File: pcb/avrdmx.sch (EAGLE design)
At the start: 15 parts, among them U1 ARDUINO_SHIELDLABEL

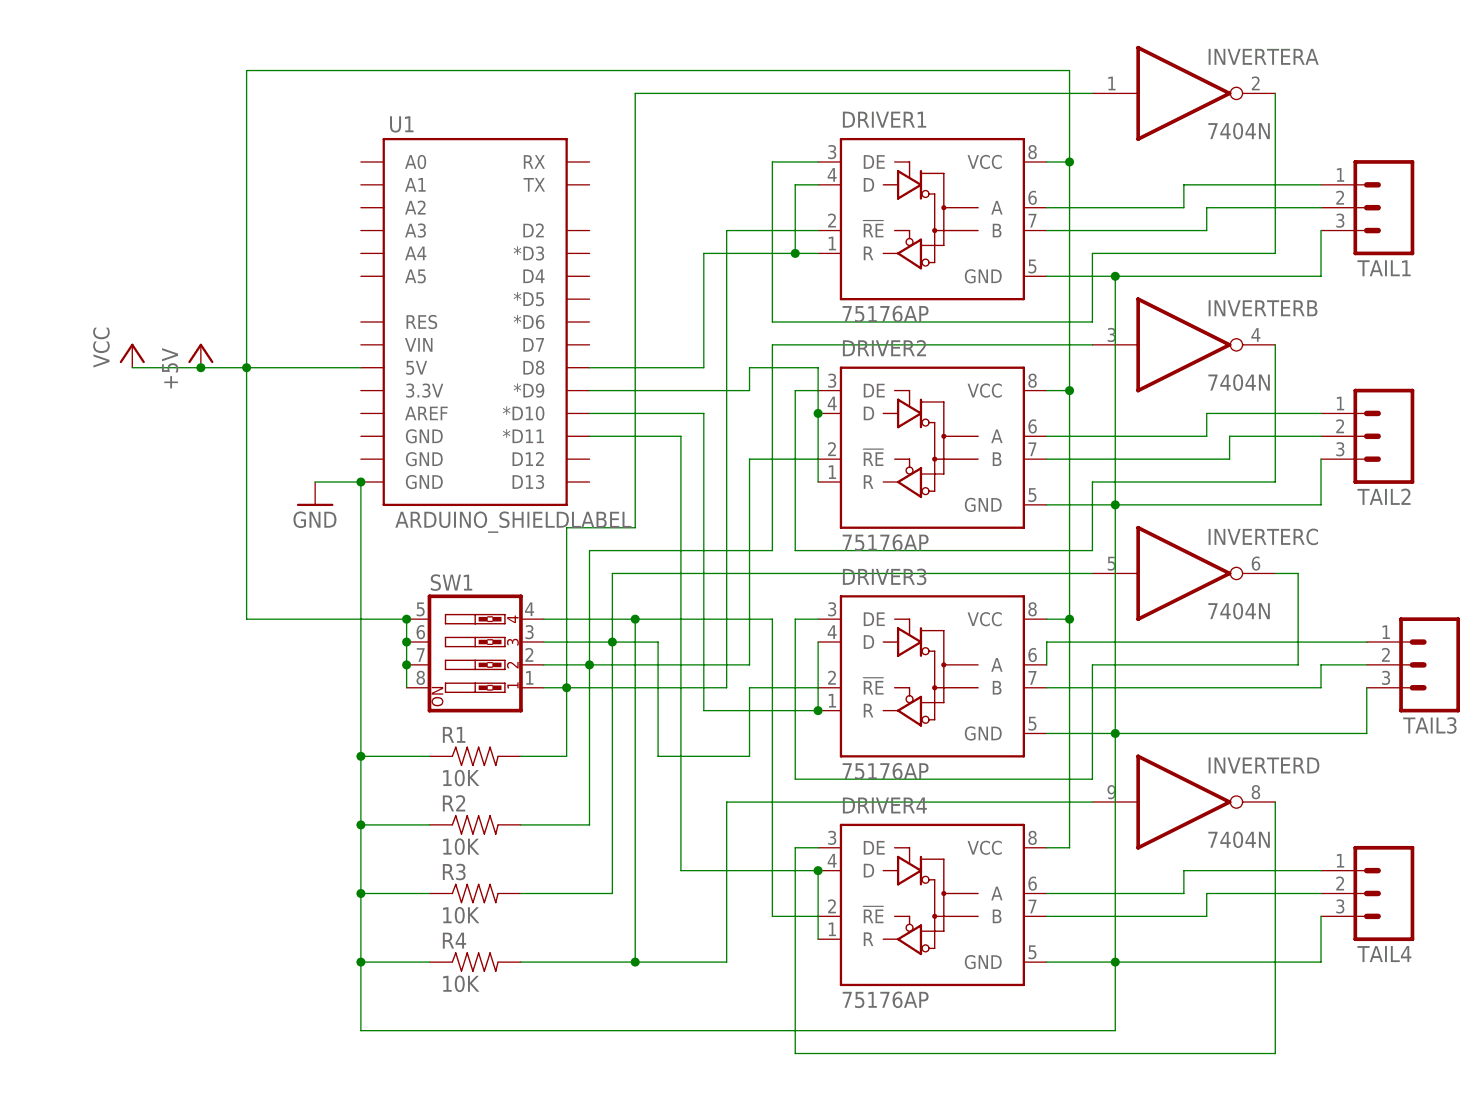
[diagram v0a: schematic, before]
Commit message: schematic changes from a long time ago, not sure if they're good
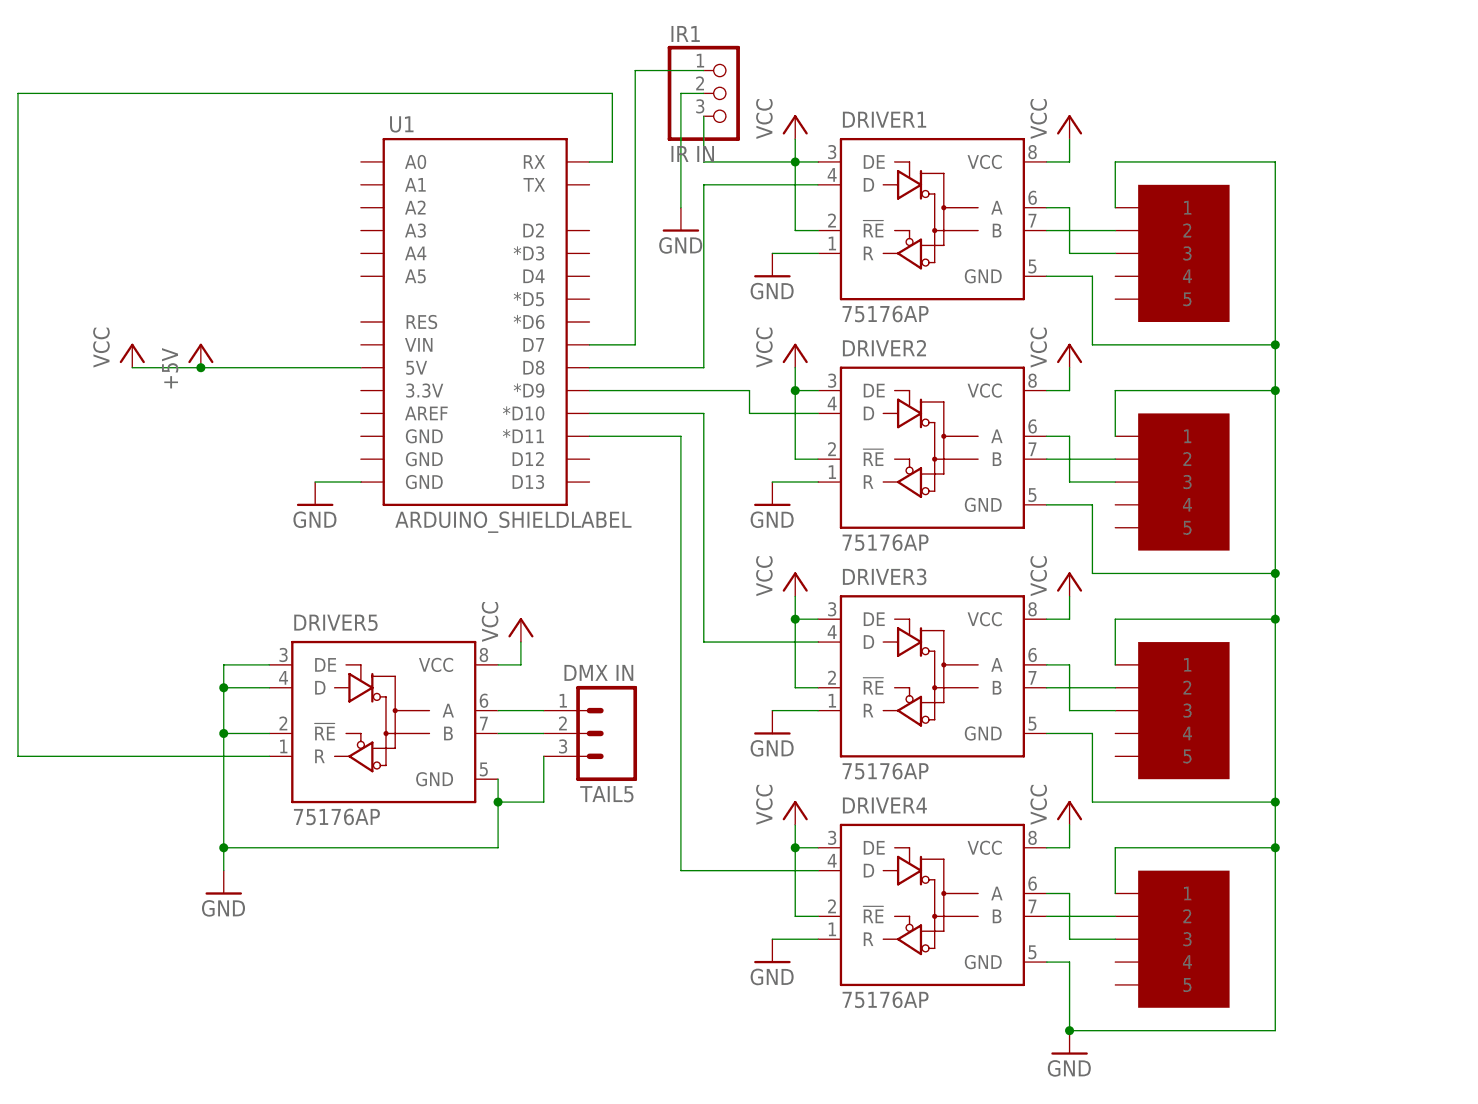
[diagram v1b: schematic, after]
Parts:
- removed INVERTER: 7404N, 74xx-us:7404N
- removed R1, R2, R3, R4: 10K, SparkFun-Resistors:RESISTORPTH-1/4W
- removed SW1: (no value), special:SW_DIP-4
- removed TAIL1, TAIL2, TAIL3, TAIL4: (no value), SparkFun-Connectors:M03-SCREW-5MM
- added DRIVER5: 75176AP, 751xx:75176AP
- added IR1: IR IN, pinhead:PINHD-1X3
- added OUT1, OUT2, OUT3, OUT4: NC5FAV, avrdmx:NC5FAV
- added TAIL5: DMX IN, SparkFun-Connectors:M03-SCREW-5MM
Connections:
- removed net N$17: DRIVER2.A, TAIL2.1
- removed net N$18: DRIVER2.B, TAIL2.2
- removed net N$19: DRIVER3.A, TAIL3.1
- removed net N$20: DRIVER3.B, TAIL3.2
- removed net N$21: DRIVER4.A, TAIL4.1
- removed net N$22: DRIVER4.B, TAIL4.2
- new net N$15: DRIVER4.A, OUT4.3
- new net N$6: DRIVER5.A, TAIL5.1
- net GND: now also DRIVER1.R, DRIVER2.R, DRIVER3.R, DRIVER4.R, DRIVER5.!RE, DRIVER5.D, DRIVER5.DE, DRIVER5.GND, IR1.2, OUT1.1, OUT2.1, OUT3.1, OUT4.1, TAIL5.3; no longer R1.1, R2.1, R3.1, R4.1, TAIL1.3, TAIL2.3, TAIL3.3, TAIL4.3
- net N$1: no longer DRIVER1.R
- net N$10: now also OUT1.3; no longer TAIL1.1
- net N$11: now also DRIVER2.B, OUT2.2; no longer DRIVER1.!RE, INVERTERA.I, R1.2, SW1.1
- net N$12: now also DRIVER2.A, OUT2.3; no longer DRIVER2.!RE, INVERTERB.I, R2.2, SW1.2
- net N$13: now also DRIVER3.B, OUT3.2; no longer DRIVER3.!RE, INVERTERC.I, R3.2, SW1.3
- net N$14: now also DRIVER3.A, OUT3.3; no longer DRIVER4.!RE, INVERTERD.I, R4.2, SW1.4
- net N$16: now also DRIVER4.B, OUT4.2; no longer DRIVER1.B, TAIL1.2
- net N$2: no longer DRIVER2.R
- net N$3: no longer DRIVER3.R
- net N$4: no longer DRIVER4.R
- net N$5: now also IR1.1, U1.D7; no longer DRIVER4.DE, INVERTERD.O
- net N$7: now also DRIVER5.B, TAIL5.2; no longer DRIVER3.DE, INVERTERC.O
- net N$8: now also DRIVER1.B, OUT1.2; no longer DRIVER2.DE, INVERTERB.O
- net N$9: now also DRIVER5.R, U1.RX; no longer DRIVER1.DE, INVERTERA.O
- net VCC: now also DRIVER1.!RE, DRIVER1.DE, DRIVER2.!RE, DRIVER2.DE, DRIVER3.!RE, DRIVER3.DE, DRIVER4.!RE, DRIVER4.DE, DRIVER5.VCC, IR1.3; no longer SW1.5, SW1.6, SW1.7, SW1.8
